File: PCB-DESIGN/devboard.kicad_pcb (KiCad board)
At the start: 2 copper layers, 21 x 51 mm, 44 parts, among them J1 USB_C_Receptacle_USB2.0_14P, J2 Conn_01x20, J3 Conn_01x20, J4 Conn_01x03, SW1 SW_Push, U1 RP2040, U2 MCP1700x-330xxTT, U3 W25Q16JVUXIQ TR, U4 TMP112xxDRL, Y1 12 MHz

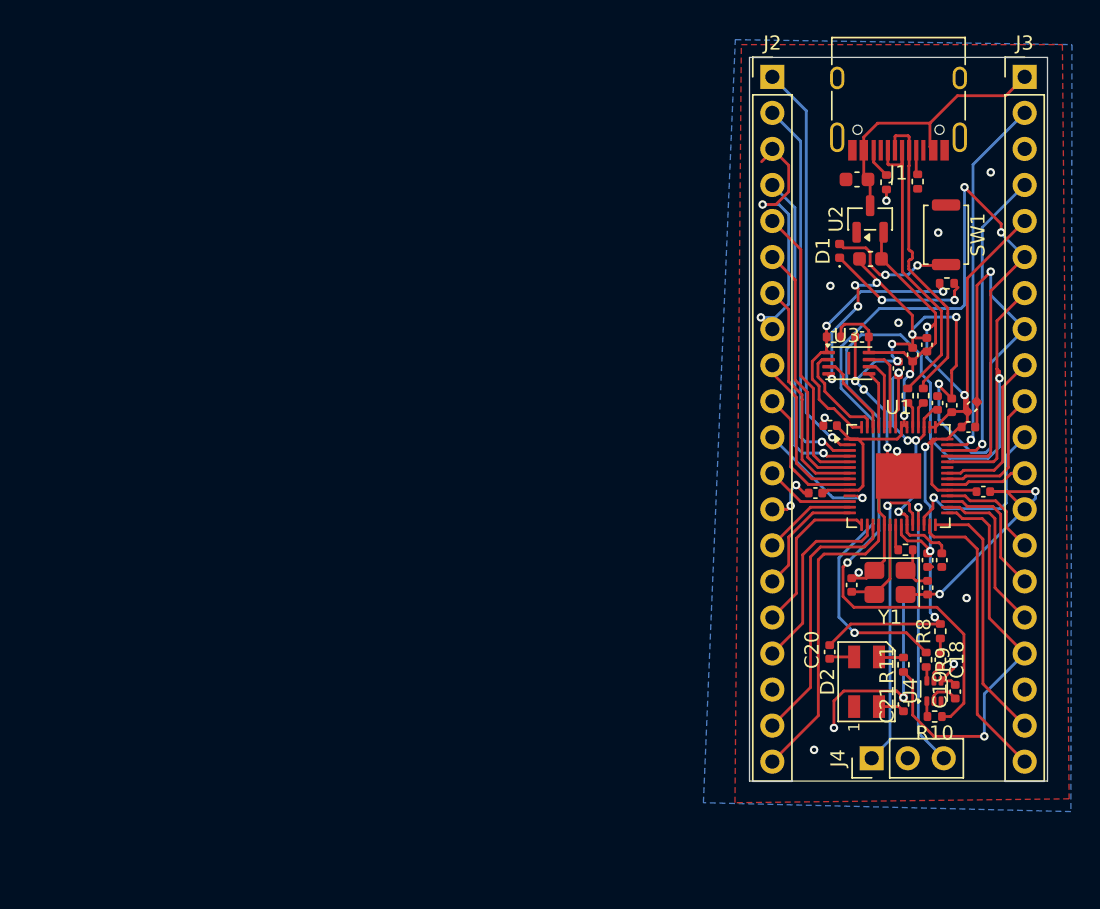
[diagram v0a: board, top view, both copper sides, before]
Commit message: Add files via upload
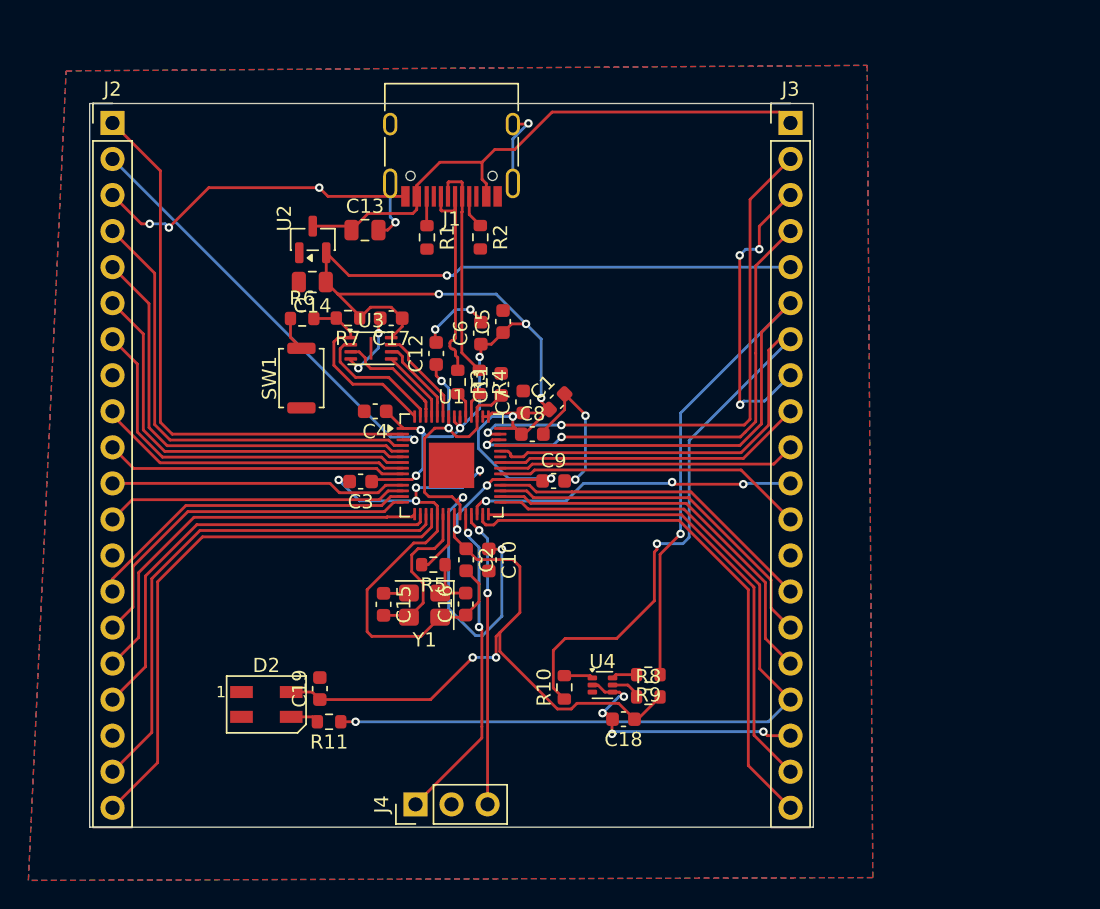
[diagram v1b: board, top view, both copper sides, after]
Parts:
- removed C20, C21: 0.1uF, Capacitor_SMD:C_0402_1005Metric
- removed D1: LED, LED_SMD:LED_0402_1005Metric
- C1, C10, C11, C12, C15, C16, C17, C2, C3, C4, C5, C6, C7, C8, C9: footprint Capacitor_SMD:C_0402_1005Metric -> Capacitor_SMD:C_0603_1608Metric
- C13, C14: footprint Capacitor_SMD:C_0603_1608Metric -> Capacitor_SMD:C_0805_2012Metric
- C18, C19: value 0.1uF -> 10uF; footprint Capacitor_SMD:C_0402_1005Metric -> Capacitor_SMD:C_0603_1608Metric
- R1, R10, R11, R2, R3, R4, R5, R6, R7, R8, R9: footprint Resistor_SMD:R_0402_1005Metric -> Resistor_SMD:R_0603_1608Metric
- moved J2 46.6 mm to (104.6, 51.4)
- moved SW1 46.5 mm to (117.9, 69.3), turned to 90 degrees
- moved R6 45.5 mm to (118.0, 65.2), turned to 0 degrees
- moved C19 44.8 mm to (119.2, 91.2)
- moved C3 43.0 mm to (122.1, 76.6), turned to 180 degrees
- moved D2 42.3 mm to (115.5, 92.3), turned to 0 degrees
- moved R11 40.7 mm to (119.9, 93.6), turned to 180 degrees
- moved C14 39.4 mm to (118.7, 62.6)
- moved U2 39.3 mm to (118.7, 59.6)
- moved C4 38.1 mm to (123.1, 71.7), turned to 180 degrees
- moved C5 35.9 mm to (132.1, 65.4), turned to 90 degrees
- moved C2 35.8 mm to (129.5, 82.2), turned to -90 degrees
- moved C6 35.3 mm to (130.6, 66.2), turned to 90 degrees
- moved C13 34.9 mm to (122.4, 58.9), turned to 0 degrees
- moved R7 34.3 mm to (121.2, 65.1)
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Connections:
- C18 pad 1: Net-(C18-Pad1) -> +3V3
- C18 pad 2: Net-(U4-V+) -> GND
- C19 pad 1: Net-(U4-GND) -> +3V3
- D2 pad 2: Net-(D2-VSS) -> GND
- D2 pad 4: Net-(D2-VDD) -> +3V3
- R6 pad 1: Net-(D1-K) -> Net-(R6-Pad1)
- R8 pad 1: Net-(C18-Pad1) -> Net-(U4-V+)
- SW1 pad 2: Net-(D1-A) -> Net-(R6-Pad1)
- U4 pad 2: Net-(U4-GND) -> GND
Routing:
- net +3V3: track 99.6 -> 166.1 mm, vias 7 -> 14
- net GPIO18: track 29.4 -> 62.0 mm
- net VBUS: track 20.1 -> 41.1 mm
- net GPIO13: track 13.7 -> 31.6 mm
- net GPIO15: track 21.5 -> 39.1 mm
- net GPIO14: track 18.9 -> 36.4 mm
- net GPIO16: track 20.8 -> 38.1 mm
- net GPIO11: track 8.61 -> 25.9 mm
- net GPIO10: track 6.57 -> 23.7 mm
- net +1V1: track 23.8 -> 40.6 mm
- net GPIO17: track 18.1 -> 34.9 mm
- net GPIO12: track 11.5 -> 28.3 mm
- net GPIO22: track 5.78 -> 22.0 mm
- net GPIO19: track 11.5 -> 27.6 mm
- net GPIO20: track 9.57 -> 25.6 mm
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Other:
- board size 21 x 51 mm -> 51 x 51 mm
- board text removed: "@urgeny99"
